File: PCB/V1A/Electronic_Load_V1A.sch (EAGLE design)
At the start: 139 parts, among them IC201 OPA77P, IC202 OPA77P, IC203 OPA77P, IC204 OPA77P, IC205 OPA77P, IC301 MAX743CPE, IC302 7805T, IC303 7805T, J101 +, J102 -, J103 +, J104 -, Q101 SIRC10DP, Q102 SIRC10DP, Q103 SIRC10DP, Q104 IXTK102N65X2PADUP-, Q105 SIRC10DP, Q106 SIRC10DP, Q107 SIRC10DP, Q108 IXTK102N65X2PADUP, U201 LTC1865-MSOP, U202 LTC1865-MSOP, U203 LTC1865-MSOP, U401 AD420, U402 AD420, U403 LT1014

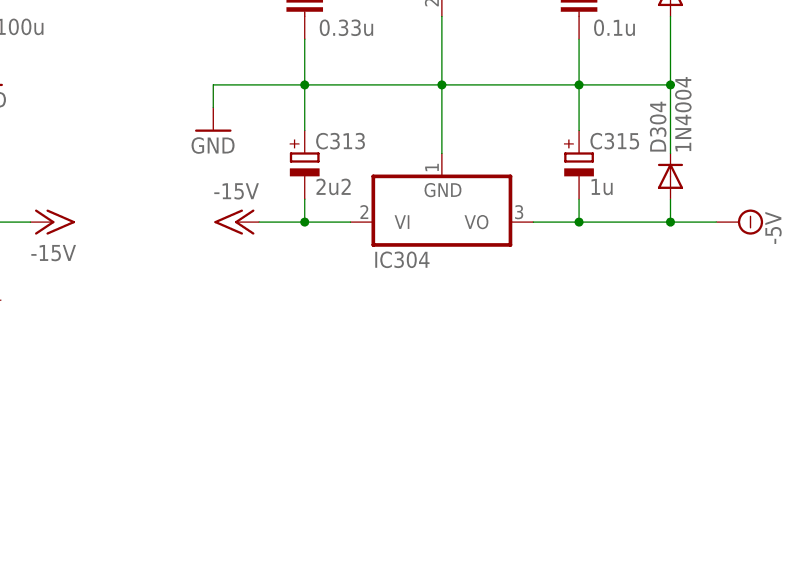
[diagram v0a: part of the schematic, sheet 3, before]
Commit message: Board layout work
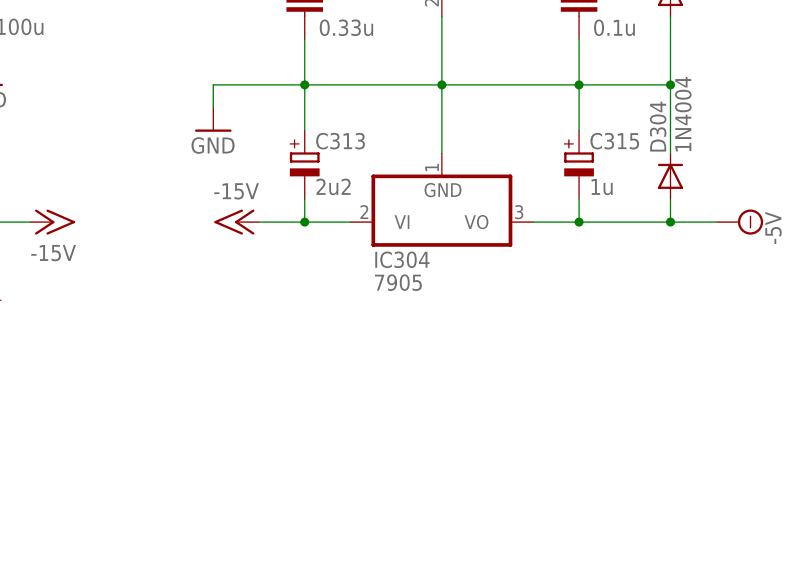
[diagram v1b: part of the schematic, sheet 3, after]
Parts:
- IC304: value (none) -> 7905
- R101, R102, R103, R104, R105, R109, R110, R111, R112: device rcl:R-EU_M5923 -> rcl:R-EU_R1206
- R107, R114: device rcl:R-EU_R0805 -> rcl:R-EU_R1206
- R403, R404, R405, R406, R407, R408, R409, R410: device rcl:R-EU_M5923 -> rcl:R-EU_R0805
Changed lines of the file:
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@@
 <?xml version="1.0" encoding="utf-8"?>
 <!DOCTYPE eagle SYSTEM "eagle.dtd">
-<eagle version="9.0.0">
+<eagle version="9.0.1">
 <drawing>
 <settings>
@@
 <part name="GND410" library="supply1" library_urn="urn:adsk.eagle:library:371" deviceset="GND" device=""/>
 <part name="GND411" library="supply1" library_urn="urn:adsk.eagle:library:371" deviceset="GND" device=""/>
-<part name="R407" library="rcl" library_urn="urn:adsk.eagle:library:334" deviceset="R-EU_" device="M5923" package3d_urn="urn:adsk.eagle:package:23564/1" value="5k"/>
-<part name="R409" library="rcl" library_urn="urn:adsk.eagle:library:334" deviceset="R-EU_" device="M5923" package3d_urn="urn:adsk.eagle:package:23564/1" value="5k"/>
-<part name="R408" library="rcl" library_urn="urn:adsk.eagle:library:334" deviceset="R-EU_" device="M5923" package3d_urn="urn:adsk.eagle:package:23564/1" value="5k"/>
-<part name="R410" library="rcl" library_urn="urn:adsk.eagle:library:334" deviceset="R-EU_" device="M5923" package3d_urn="urn:adsk.eagle:package:23564/1" value="5k"/>
-<part name="R405" library="rcl" library_urn="urn:adsk.eagle:library:334" deviceset="R-EU_" device="M5923" package3d_urn="urn:adsk.eagle:package:23564/1" value="100R"/>
+<part name="R407" library="rcl" library_urn="urn:adsk.eagle:library:334" deviceset="R-EU_" device="R0805" package3d_urn="urn:adsk.eagle:package:23553/2" value="5k"/>
+<part name="R409" library="rcl" library_urn="urn:adsk.eagle:library:334" deviceset="R-EU_" device="R0805" package3d_urn="urn:adsk.eagle:package:23553/2" value="5k"/>
+<part name="R408" library="rcl" library_urn="urn:adsk.eagle:library:334" deviceset="R-EU_" device="R0805" package3d_urn="urn:adsk.eagle:package:23553/2" value="5k"/>
+<part name="R410" library="rcl" library_urn="urn:adsk.eagle:library:334" deviceset="R-EU_" device="R0805" package3d_urn="urn:adsk.eagle:package:23553/2" value="5k"/>
+<part name="R405" library="rcl" library_urn="urn:adsk.eagle:library:334" deviceset="R-EU_" device="R0805" package3d_urn="urn:adsk.eagle:package:23553/2" value="100R"/>
 <part name="R401" library="rcl" library_urn="urn:adsk.eagle:library:334" deviceset="R-TRIMM" device="4G/J" package3d_urn="urn:adsk.eagle:package:23728/1" value="20k"/>
-<part name="R403" library="rcl" library_urn="urn:adsk.eagle:library:334" deviceset="R-EU_" device="M5923" package3d_urn="urn:adsk.eagle:package:23564/1" value="200k"/>
-<part name="R406" library="rcl" library_urn="urn:adsk.eagle:library:334" deviceset="R-EU_" device="M5923" package3d_urn="urn:adsk.eagle:package:23564/1" value="100R"/>
-<part name="R404" library="rcl" library_urn="urn:adsk.eagle:library:334" deviceset="R-EU_" device="M5923" package3d_urn="urn:adsk.eagle:package:23564/1" value="200k"/>
+<part name="R403" library="rcl" library_urn="urn:adsk.eagle:library:334" deviceset="R-EU_" device="R0805" package3d_urn="urn:adsk.eagle:package:23553/2" value="200k"/>
+<part name="R406" library="rcl" library_urn="urn:adsk.eagle:library:334" deviceset="R-EU_" device="R0805" package3d_urn="urn:adsk.eagle:package:23553/2" value="100R"/>
+<part name="R404" library="rcl" library_urn="urn:adsk.eagle:library:334" deviceset="R-EU_" device="R0805" package3d_urn="urn:adsk.eagle:package:23553/2" value="200k"/>
 <part name="R402" library="rcl" library_urn="urn:adsk.eagle:library:334" deviceset="R-TRIMM" device="4G/J" package3d_urn="urn:adsk.eagle:package:23728/1" value="20k"/>
 <part name="GND409" library="supply1" library_urn="urn:adsk.eagle:library:371" deviceset="GND" device=""/>
@@
 <part name="P-401" library="supply1" library_urn="urn:adsk.eagle:library:371" deviceset="-15V" device=""/>
 <part name="IC303" library="linear" library_urn="urn:adsk.eagle:library:262" deviceset="78*" device="T" package3d_urn="urn:adsk.eagle:package:16414/1" technology="05"/>
-<part name="IC304" library="linear" library_urn="urn:adsk.eagle:library:262" deviceset="79*" device="T" package3d_urn="urn:adsk.eagle:package:16414/1" technology="05"/>
+<part name="IC304" library="linear" library_urn="urn:adsk.eagle:library:262" deviceset="79*" device="T" package3d_urn="urn:adsk.eagle:package:16414/1" technology="05" value="7905"/>
 <part name="C307" library="rcl" library_urn="urn:adsk.eagle:library:334" deviceset="C-EU" device="C0805" package3d_urn="urn:adsk.eagle:package:23617/2" value="0.33u"/>
 <part name="C308" library="rcl" library_urn="urn:adsk.eagle:library:334" deviceset="C-EU" device="C0805" package3d_urn="urn:adsk.eagle:package:23617/2" value="0.1u"/>
@@
 <part name="J102" library="SparkFun-Connectors" deviceset="BANANA_CONN" device="" value="-"/>
 <part name="S101" library="switch" library_urn="urn:adsk.eagle:library:380" deviceset="320-938" device="" package3d_urn="urn:adsk.eagle:package:27685/1"/>
-<part name="R104" library="rcl" library_urn="urn:adsk.eagle:library:334" deviceset="R-EU_" device="M5923" package3d_urn="urn:adsk.eagle:package:23564/1" value="100R"/>
-<part name="R111" library="rcl" library_urn="urn:adsk.eagle:library:334" deviceset="R-EU_" device="M5923" package3d_urn="urn:adsk.eagle:package:23564/1" value="100R"/>
-<part name="R101" library="rcl" library_urn="urn:adsk.eagle:library:334" deviceset="R-EU_" device="M5923" package3d_urn="urn:adsk.eagle:package:23564/1" value="100R"/>
-<part name="R103" library="rcl" library_urn="urn:adsk.eagle:library:334" deviceset="R-EU_" device="M5923" package3d_urn="urn:adsk.eagle:package:23564/1" value="100R"/>
-<part name="R105" library="rcl" library_urn="urn:adsk.eagle:library:334" deviceset="R-EU_" device="M5923" package3d_urn="urn:adsk.eagle:package:23564/1" value="100R"/>
-<part name="R107" library="rcl" library_urn="urn:adsk.eagle:library:334" deviceset="R-EU_" device="R0805" package3d_urn="urn:adsk.eagle:package:23553/2" value="2R"/>
+<part name="R104" library="rcl" library_urn="urn:adsk.eagle:library:334" deviceset="R-EU_" device="R1206" package3d_urn="urn:adsk.eagle:package:23540/2" value="100R"/>
+<part name="R111" library="rcl" library_urn="urn:adsk.eagle:library:334" deviceset="R-EU_" device="R1206" package3d_urn="urn:adsk.eagle:package:23540/2" value="100R"/>
+<part name="R101" library="rcl" library_urn="urn:adsk.eagle:library:334" deviceset="R-EU_" device="R1206" package3d_urn="urn:adsk.eagle:package:23540/2" value="100R"/>
+<part name="R103" library="rcl" library_urn="urn:adsk.eagle:library:334" deviceset="R-EU_" device="R1206" package3d_urn="urn:adsk.eagle:package:23540/2" value="100R"/>
+<part name="R105" library="rcl" library_urn="urn:adsk.eagle:library:334" deviceset="R-EU_" device="R1206" package3d_urn="urn:adsk.eagle:package:23540/2" value="100R"/>
+<part name="R107" library="rcl" library_urn="urn:adsk.eagle:library:334" deviceset="R-EU_" device="R1206" package3d_urn="urn:adsk.eagle:package:23540/2" value="2R"/>
 <part name="R106" library="rcl" library_urn="urn:adsk.eagle:library:334" deviceset="R-EU_" device="R6332" package3d_urn="urn:adsk.eagle:package:23559/2" value="0R004"/>
-<part name="R110" library="rcl" library_urn="urn:adsk.eagle:library:334" deviceset="R-EU_" device="M5923" package3d_urn="urn:adsk.eagle:package:23564/1" value="100R"/>
-<part name="R112" library="rcl" library_urn="urn:adsk.eagle:library:334" deviceset="R-EU_" device="M5923" package3d_urn="urn:adsk.eagle:package:23564/1" value="100R"/>
-<part name="R114" library="rcl" library_urn="urn:adsk.eagle:library:334" deviceset="R-EU_" device="R0805" package3d_urn="urn:adsk.eagle:package:23553/2" value="2R"/>
+<part name="R110" library="rcl" library_urn="urn:adsk.eagle:library:334" deviceset="R-EU_" device="R1206" package3d_urn="urn:adsk.eagle:package:23540/2" value="100R"/>
+<part name="R112" library="rcl" library_urn="urn:adsk.eagle:library:334" deviceset="R-EU_" device="R1206" package3d_urn="urn:adsk.eagle:package:23540/2" value="100R"/>
+<part name="R114" library="rcl" library_urn="urn:adsk.eagle:library:334" deviceset="R-EU_" device="R1206" package3d_urn="urn:adsk.eagle:package:23540/2" value="2R"/>
 <part name="R113" library="rcl" library_urn="urn:adsk.eagle:library:334" deviceset="R-EU_" device="R6332" package3d_urn="urn:adsk.eagle:package:23559/2" value="0R004"/>
 <part name="GND101" library="supply1" library_urn="urn:adsk.eagle:library:371" deviceset="GND" device=""/>
@@
 <part name="Q102" library="transistors" deviceset="SIRC10DP" device=""/>
 <part name="Q103" library="transistors" deviceset="SIRC10DP" device=""/>
-<part name="R102" library="rcl" library_urn="urn:adsk.eagle:library:334" deviceset="R-EU_" device="M5923" package3d_urn="urn:adsk.eagle:package:23564/1" value="100R"/>
-<part name="R109" library="rcl" library_urn="urn:adsk.eagle:library:334" deviceset="R-EU_" device="M5923" package3d_urn="urn:adsk.eagle:package:23564/1" value="100R"/>
+<part name="R102" library="rcl" library_urn="urn:adsk.eagle:library:334" deviceset="R-EU_" device="R1206" package3d_urn="urn:adsk.eagle:package:23540/2" value="100R"/>
+<part name="R109" library="rcl" library_urn="urn:adsk.eagle:library:334" deviceset="R-EU_" device="R1206" package3d_urn="urn:adsk.eagle:package:23540/2" value="100R"/>
 <part name="Q105" library="transistors" deviceset="SIRC10DP" device=""/>
 <part name="Q106" library="transistors" deviceset="SIRC10DP" device=""/>
